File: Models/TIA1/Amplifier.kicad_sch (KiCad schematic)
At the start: 4 parts, among them U1 OPA828

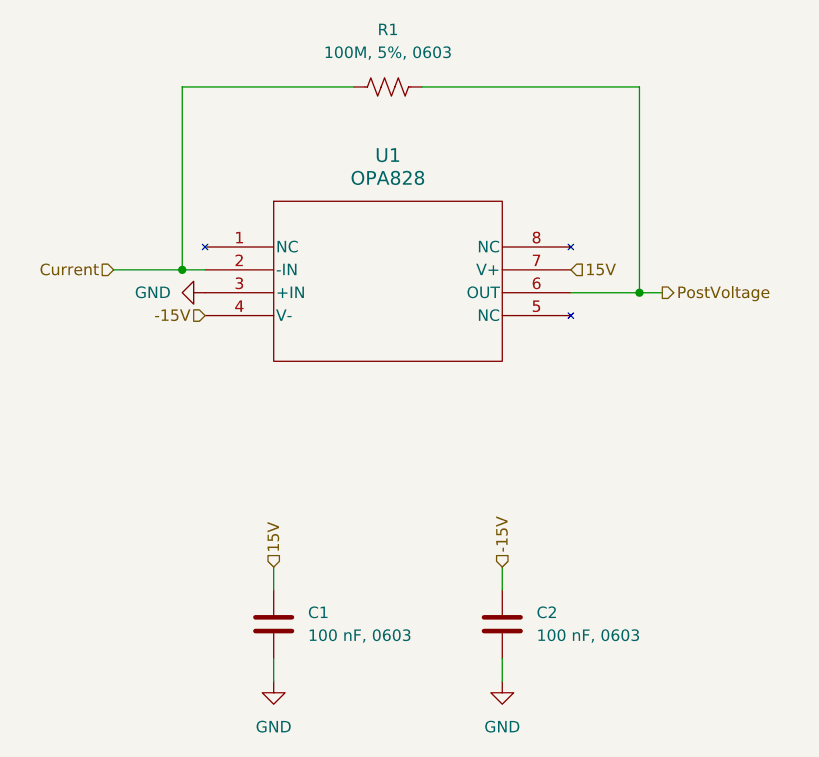
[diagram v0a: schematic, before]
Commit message: Save progress
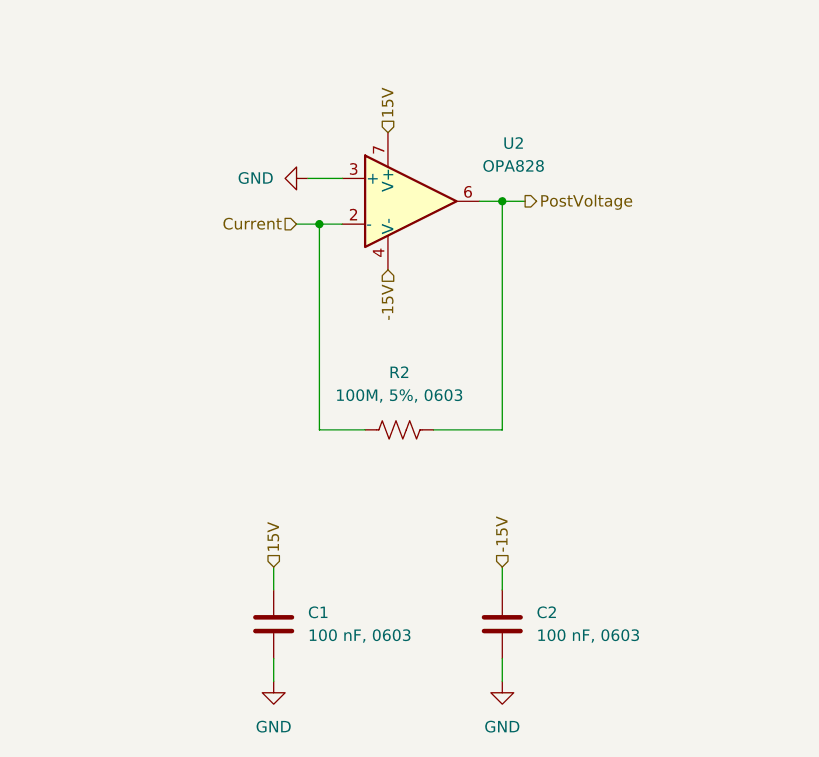
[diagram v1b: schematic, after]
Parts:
- removed R1: 100M, 5%, 0603, symbol Device:R_US
- removed U1: OPA828, symbol Vendor:OPA828
- added R2: 100M, 5%, 0603, symbol Device:R_US
- added U2: OPA828, symbol Amplifier_Operational:OP179GS
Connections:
- net -15V: now also U2.4 (V-)
- net 15V: now also U2.7 (V+)
- net Current: now also R2.1, U2.2 (-)
- net GND: now also U2.3 (+)
- net PostVoltage: now also R2.2, U2.6
